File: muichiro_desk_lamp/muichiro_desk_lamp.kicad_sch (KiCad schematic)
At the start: 12 parts, among them J1 Conn_01x03_Pin, U1 ESP32-C3-DevKitM-1

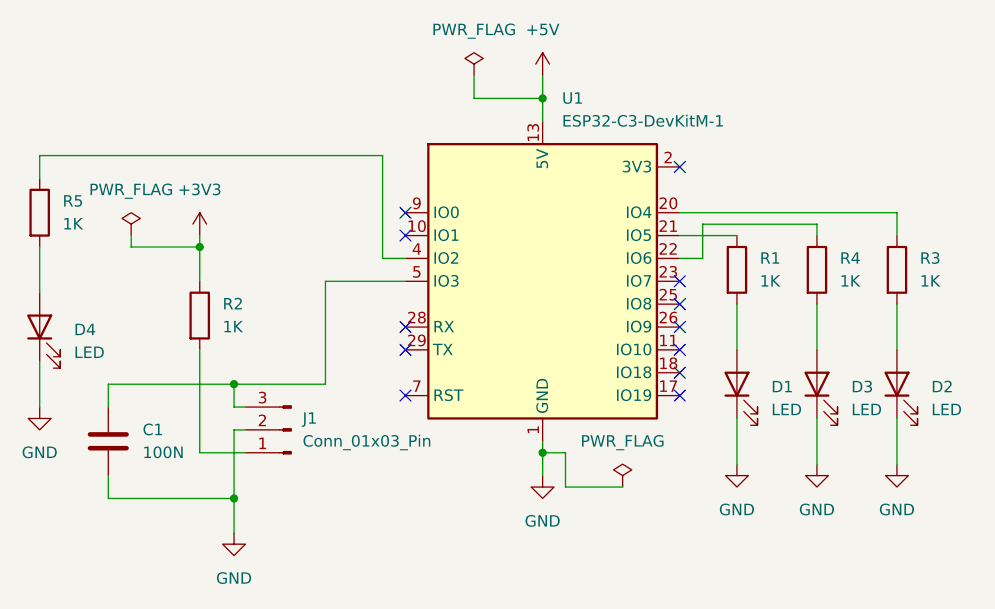
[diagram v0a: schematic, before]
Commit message: updated Tamagotchi and muichiro_desk_lamp
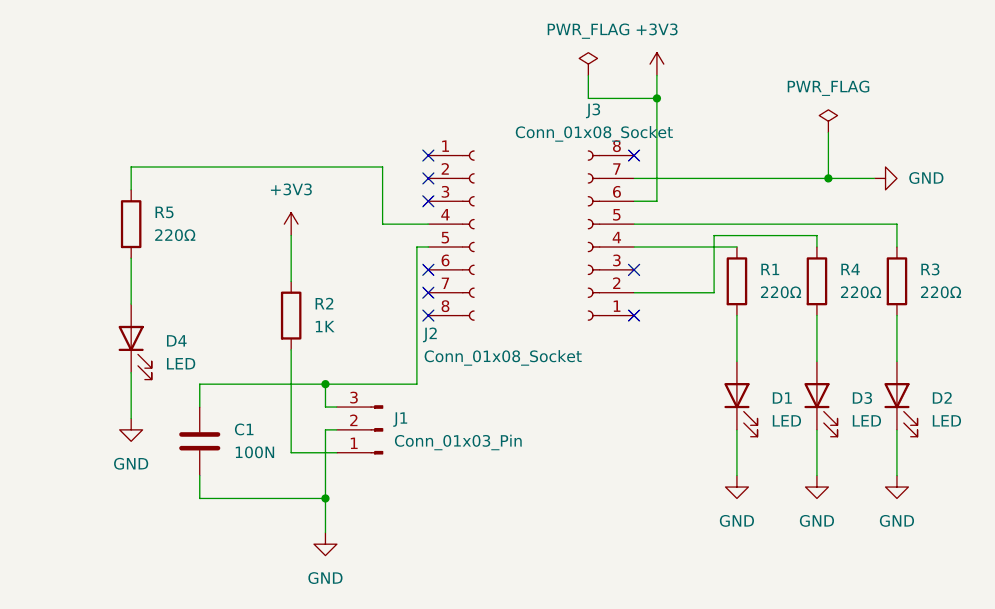
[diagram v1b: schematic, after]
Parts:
- removed U1: ESP32-C3-DevKitM-1, desk-lamp:ESP32_Socket_Dual_1x15, symbol RF_Module:ESP32-C3-DevKitM-1
- added J2, J3: Conn_01x08_Socket, Connector_PinSocket_2.54mm:PinSocket_1x08_P2.54mm_Vertical_SMD_Pin1Left, symbol Connector:Conn_01x08_Socket
- R1, R3, R4, R5: value 1K -> 220Ω
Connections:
- net +3V3: now also J3.6 (Pin_6)
- net GND: now also J3.7 (Pin_7)
- net at R1.1: now also J3.4 (Pin_4)
- net at R3.1: now also J3.5 (Pin_5)
- net at R5.1: now also J2.4 (Pin_4)
- net at R4.1: now also J3.2 (Pin_2)
- net at C1.1, J1.3 (Pin_3): now also J2.5 (Pin_5)
- no-connect marks 12 -> 9
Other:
- moved on the sheet: C1, D1, D2, D3, D4, J1, R1, R2, R3, R4, R5
